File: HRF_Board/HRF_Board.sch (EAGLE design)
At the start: 14 parts, among them U1 MAX30101EFD, Y1 ABS06-107-32.768KHZ-T

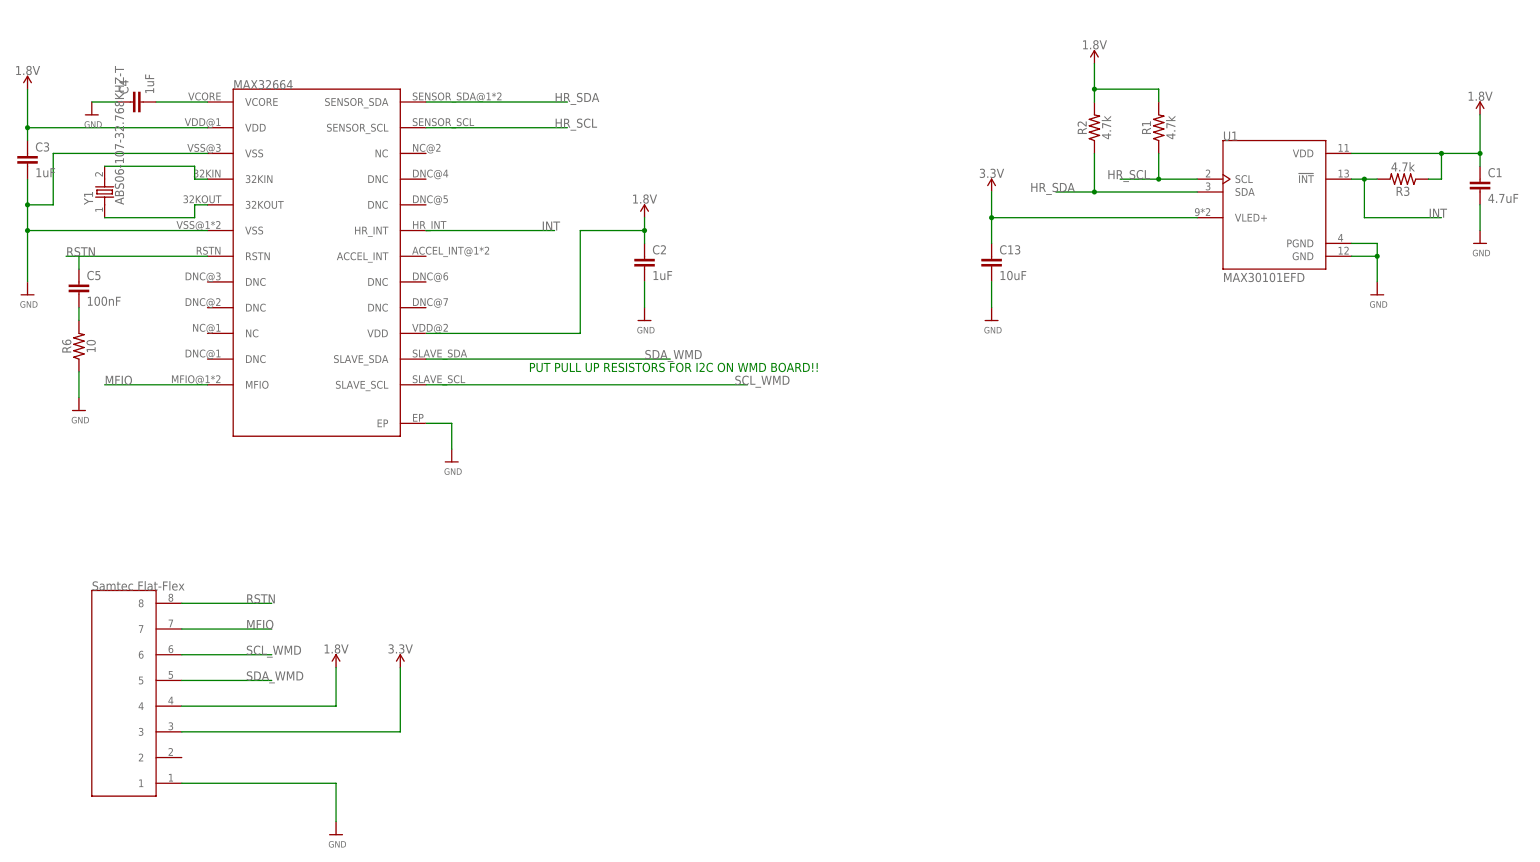
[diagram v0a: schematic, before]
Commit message: Fully routed
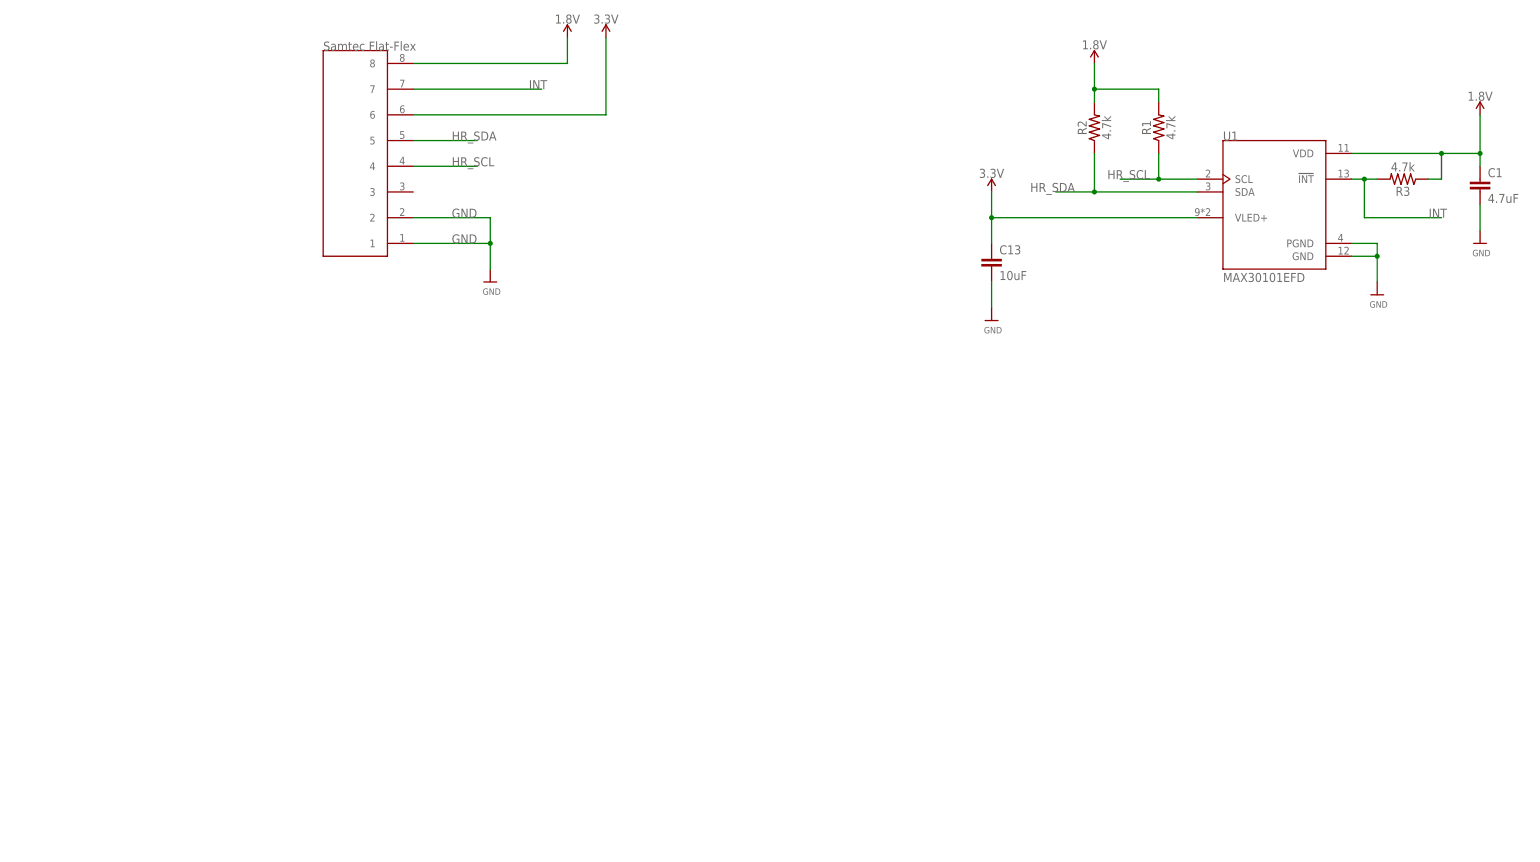
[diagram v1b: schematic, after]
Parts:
- removed C2, C3, C4: 1uF, SparkFun-Capacitors:1.0UF-0603-16V-10%
- removed C5: 100nF, SparkFun-Capacitors:1.0UF-0603-16V-10%
- removed R6: 10, SparkFun-Resistors:100KOHM-0603-1/10W-1%
- removed U$1: MAX32664_TQFN, MAX32664:MAX32664_TQFN
- removed Y1: ABS06-107-32.768KHZ-T, ABS06-107-32.768KHZ-T:ABS06-107-32.768KHZ-T
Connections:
- removed net MFIO: U$1.MFIO, U$9.7
- removed net N$1: U$1.32KIN, Y1.2
- removed net N$3: U$1.32KOUT, Y1.1
- removed net N$4: C4.2, U$1.VCORE
- removed net N$7: C5.2, R6.2
- removed net RSTN: C5.1, U$1.RSTN, U$9.8
- removed net SCL_WMD: U$1.SLAVE_SCL, U$9.6
- removed net SDA_WMD: U$1.SLAVE_SDA, U$9.5
- net 1.8V: now also U$9.8; no longer C2.1, C3.1, U$1.VDD@1, U$1.VDD@2, U$9.4
- net 3.3V: now also U$9.6; no longer U$9.3
- net GND: now also U$9.2; no longer C2.2, C3.2, C4.1, R6.1, U$1.EP, U$1.VSS@1, U$1.VSS@2
- net HR_SCL: now also U$9.4; no longer U$1.SENSOR_SCL
- net HR_SDA: now also U$9.5; no longer U$1.SENSOR_SDA
- net INT: now also U$9.7; no longer U$1.HR_INT
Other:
- note removed: "PUT PULL UP RESISTORS FOR I2C ON WMD BOARD!!"
